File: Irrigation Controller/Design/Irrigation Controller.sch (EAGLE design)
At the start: 21 parts, among them IC1 7809DT, IC2 LM1117-3.3, IC3 7805DT, U1 ESP-WROOM-32, U4 MB6S

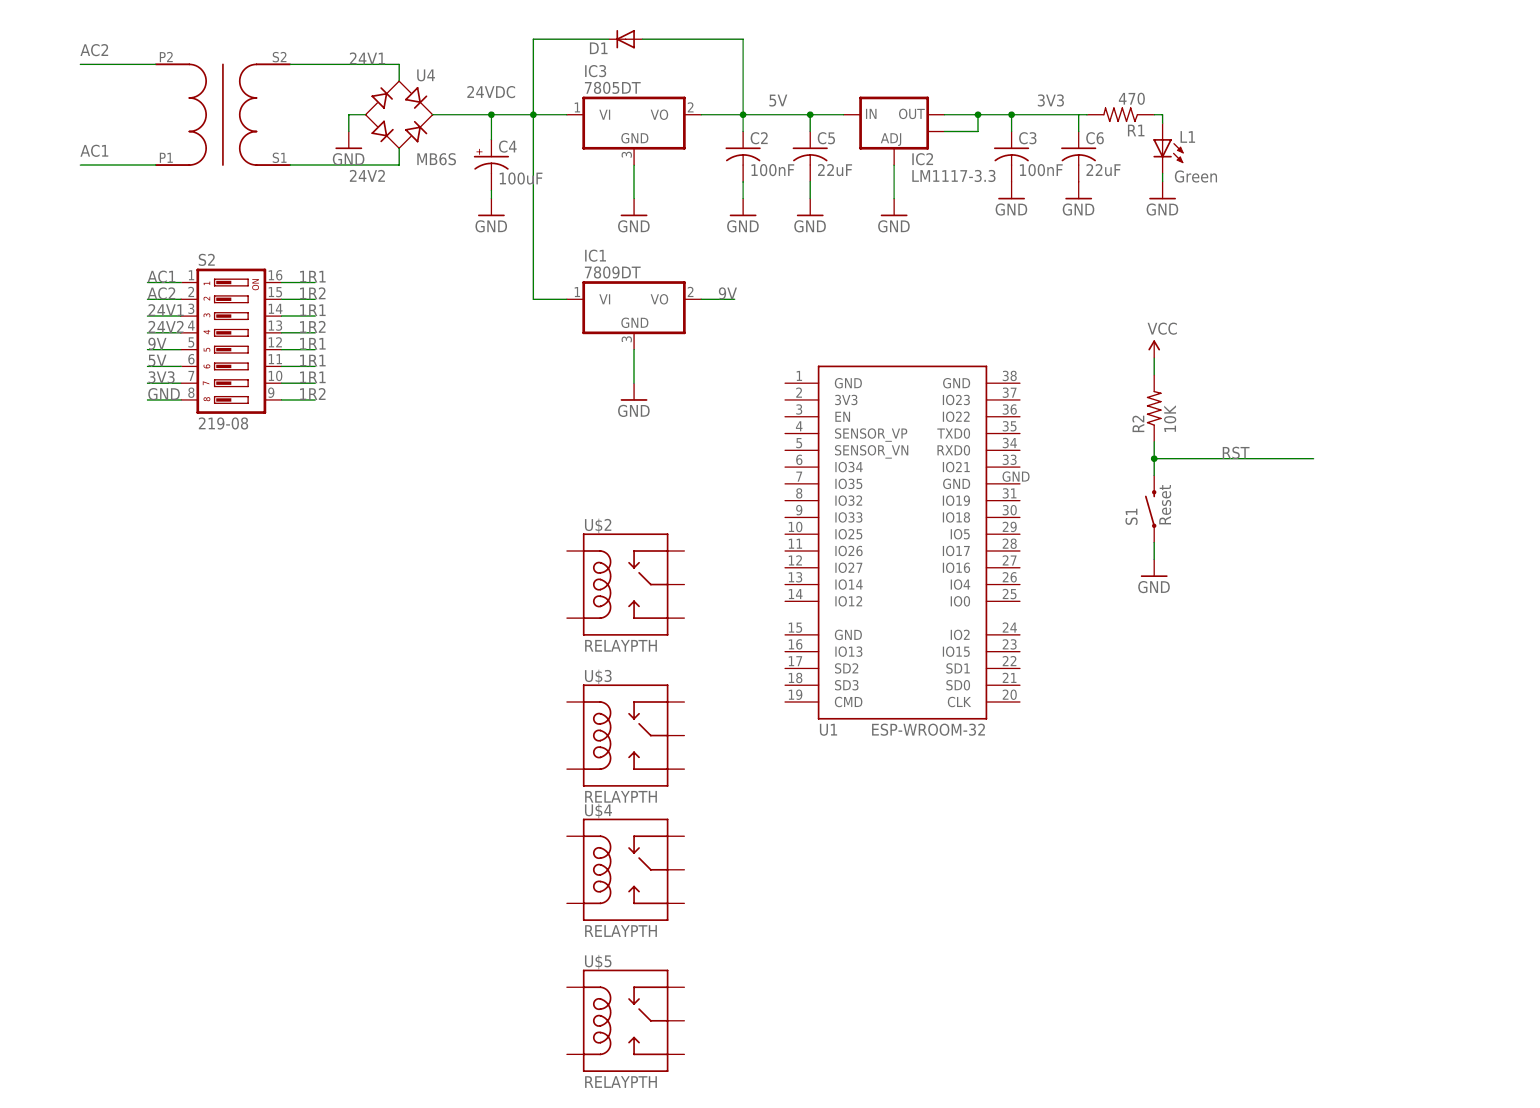
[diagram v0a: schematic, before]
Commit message: Updated Schematics and Board
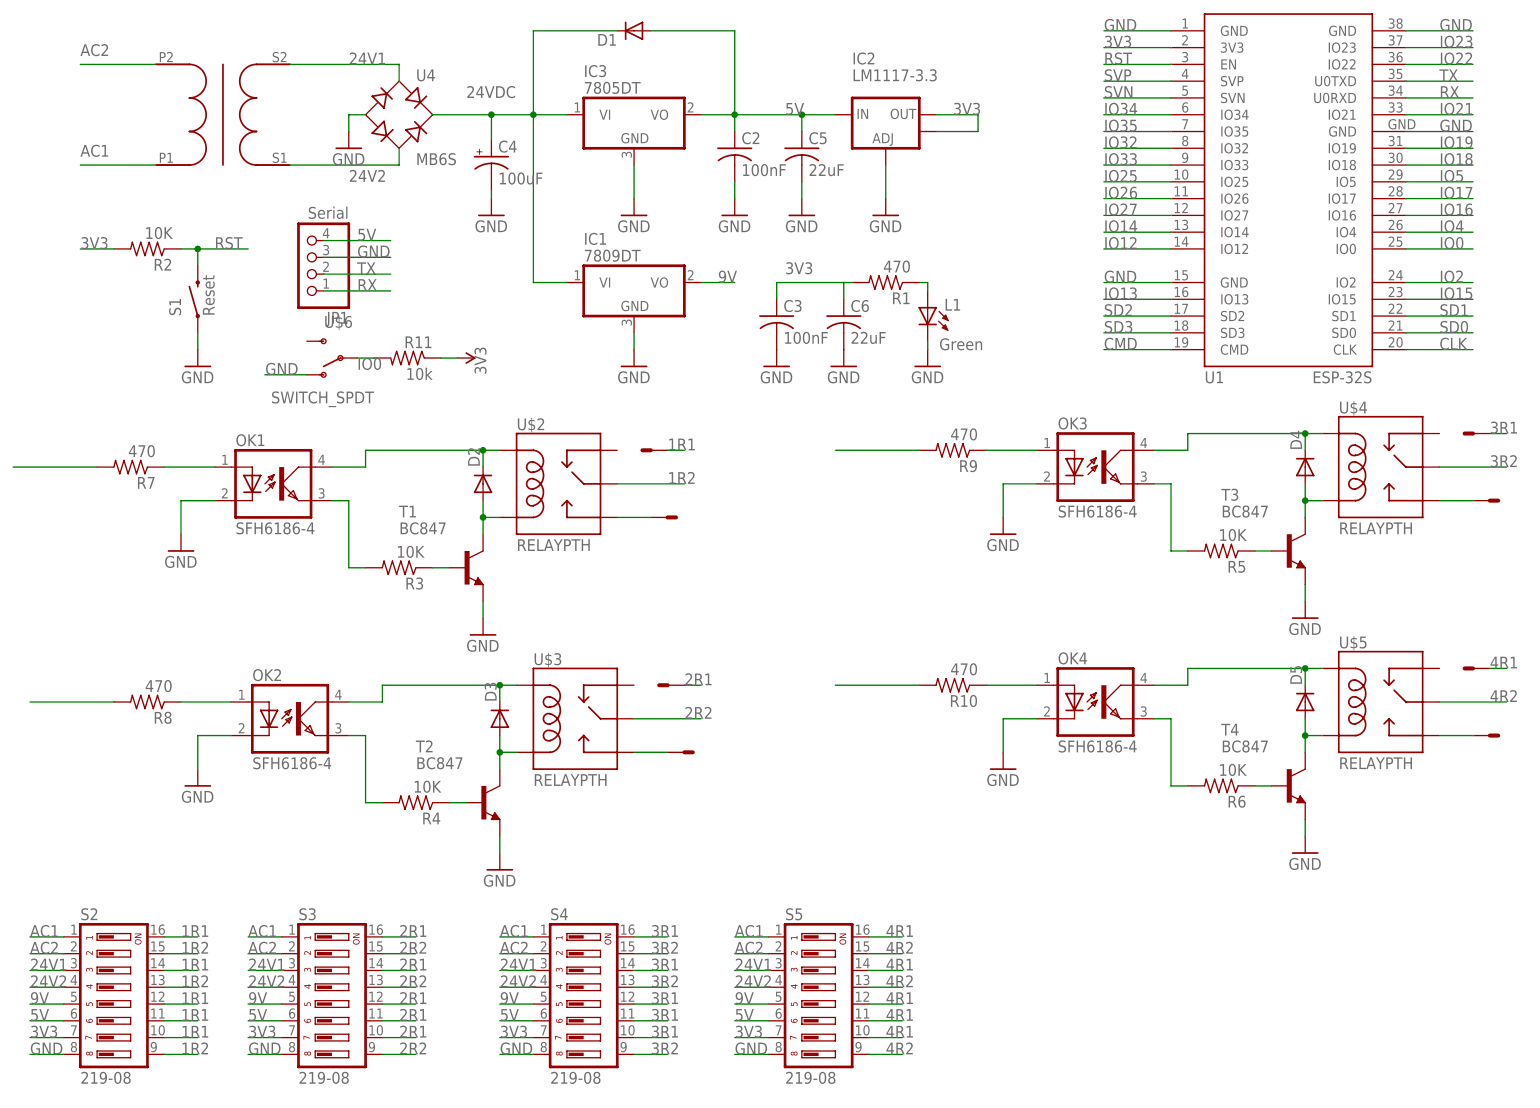
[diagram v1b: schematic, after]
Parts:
- added D2, D3, D4, D5: (no value), diode:DIODE-SOD123
- added JP1: Serial, SpaceDIY_connectors:PINHD-1X4
- added OK1, OK2, OK3, OK4: SFH6186-4, optocoupler:SFH6186-4
- added R10, R7, R8, R9: 470, resistor:R-US_R1206
- added R11: 10k, SpaceDIY_passive_components:R1206
- added R3, R4, R5, R6: 10K, resistor:R-US_R1206
- added S3, S4, S5: 219-08, switch-dil:219-08
- added T1, T2, T3, T4: BC847, transistor:BC847
- added U$6: SWITCH_SPDT, SparkFun-Retired:SWITCH_SPDT
- added X1, X2, X3, X4: 22-23-2021, con-molex:22-23-2021
- U1: value ESP-WROOM-32 -> ESP-32S; device esp32:ESP-WROOM-32 -> esp32:ESP-32S
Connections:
- removed net VCC: R2.2
- new net 2R1: S3.10, S3.11, S3.12, S3.14, S3.16, X2-1.S
- new net 2R2: S3.13, S3.15, S3.9, U$3.SWCOMMON
- new net 3R1: S4.10, S4.11, S4.12, S4.14, S4.16, X3-1.S
- new net 3R2: S4.13, S4.15, S4.9, U$4.SWCOMMON
- new net 4R1: S5.10, S5.11, S5.12, S5.14, S5.16, X4-1.S
- new net 4R2: S5.13, S5.15, S5.9, U$5.SWCOMMON
- new net CLK: U1.CLK
- new net CMD: U1.CMD
- new net IO0: R11.2, U$6.P, U1.IO0
- new net IO12: U1.IO12
- new net IO13: U1.IO13
- new net IO14: U1.IO14
- new net IO15: U1.IO15
- new net IO16: U1.IO16
- new net IO17: U1.IO17
- new net IO18: U1.IO18
- new net IO19: U1.IO19
- new net IO2: U1.IO2
- new net IO21: U1.IO21
- new net IO22: U1.IO22
- new net IO23: U1.IO23
- new net IO25: U1.IO25
- new net IO26: U1.IO26
- new net IO27: U1.IO27
- new net IO32: U1.IO32
- new net IO33: U1.IO33
- new net IO34: U1.IO34
- new net IO35: U1.IO35
- new net IO4: U1.IO4
- new net IO5: U1.IO5
- new net N$1: U$5.SWOPEN, X4-2.S
- new net N$10: D3.C, OK2.COL, U$3.COIL1
- new net N$11: D3.A, T2.C, U$3.COIL0
- new net N$12: OK2.EMIT, R4.2
- new net N$13: R4.1, T2.B
- new net N$14: D4.C, OK3.COL, U$4.COIL1
- new net N$15: D4.A, T3.C, U$4.COIL0
- new net N$16: OK3.EMIT, R5.2
- new net N$17: R5.1, T3.B
- new net N$18: D5.C, OK4.COL, U$5.COIL1
- new net N$19: D5.A, T4.C, U$5.COIL0
- new net N$2: U$4.SWOPEN, X3-2.S
- new net N$20: OK4.EMIT, R6.2
- new net N$21: R6.1, T4.B
- new net N$22: OK1.A, R7.1
- new net N$23: R7.2
- new net N$25: OK2.A, R8.1
- new net N$26: R8.2
- new net N$27: OK3.A, R9.1
- new net N$28: R9.2
- new net N$29: OK4.A, R10.1
- new net N$30: R10.2
- new net N$4: U$3.SWOPEN, X2-2.S
- new net N$5: U$2.SWOPEN, X1-2.S
- new net N$6: D2.C, OK1.COL, U$2.COIL1
- new net N$7: D2.A, T1.C, U$2.COIL0
- new net N$8: OK1.EMIT, R3.2
- new net N$9: R3.1, T1.B
- new net RX: JP1.1, U1.U0RXD
- new net SD0: U1.SD0
- new net SD1: U1.SD1
- new net SD2: U1.SD2
- new net SD3: U1.SD3
- new net SVN: U1.SVN
- new net SVP: U1.SVP
- new net TX: JP1.2, U1.U0TXD
- net 1R1: now also X1-1.S
- net 1R2: now also U$2.SWCOMMON
- net 24V1: now also S3.3, S4.3, S5.3
- net 24V2: now also S3.4, S4.4, S5.4
- net 3V3: now also R11.1, R2.2, S3.7, S4.7, S5.7, U1.3V3
- net 5V: now also JP1.4, S3.6, S4.6, S5.6
- net 9V: now also S3.5, S4.5, S5.5
- net AC1: now also S3.1, S4.1, S5.1
- net AC2: now also S3.2, S4.2, S5.2
- net GND: now also JP1.3, OK1.C, OK2.C, OK3.C, OK4.C, S3.8, S4.8, S5.8, T1.E, T2.E, T3.E, T4.E, U$6.O, U1.GND@1, U1.GND@2, U1.GND@3, U1.GND@4
- net RST: now also U1.EN
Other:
- moved on the sheet: C2, C3, C5, C6, D1, IC1, IC2, L1, R1, R2, S1, S2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
